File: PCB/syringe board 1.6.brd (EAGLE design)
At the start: 68.6 x 30.5 mm, 40 parts, among them IC1 A3967SLB, Q1 RESONATOR_CSTCE_V, U1 ATMEGA328P_TQFP, U2 PCA9306

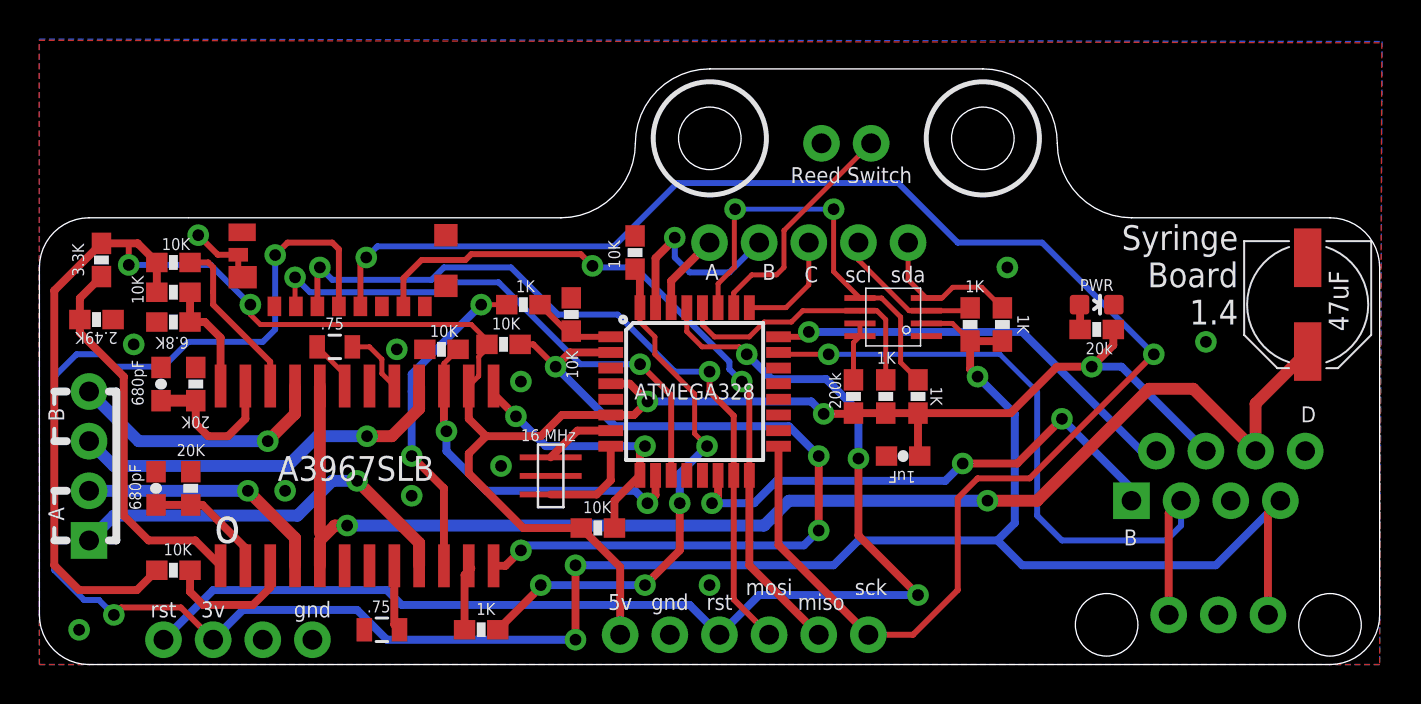
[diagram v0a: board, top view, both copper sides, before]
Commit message: PCB update to 1.6
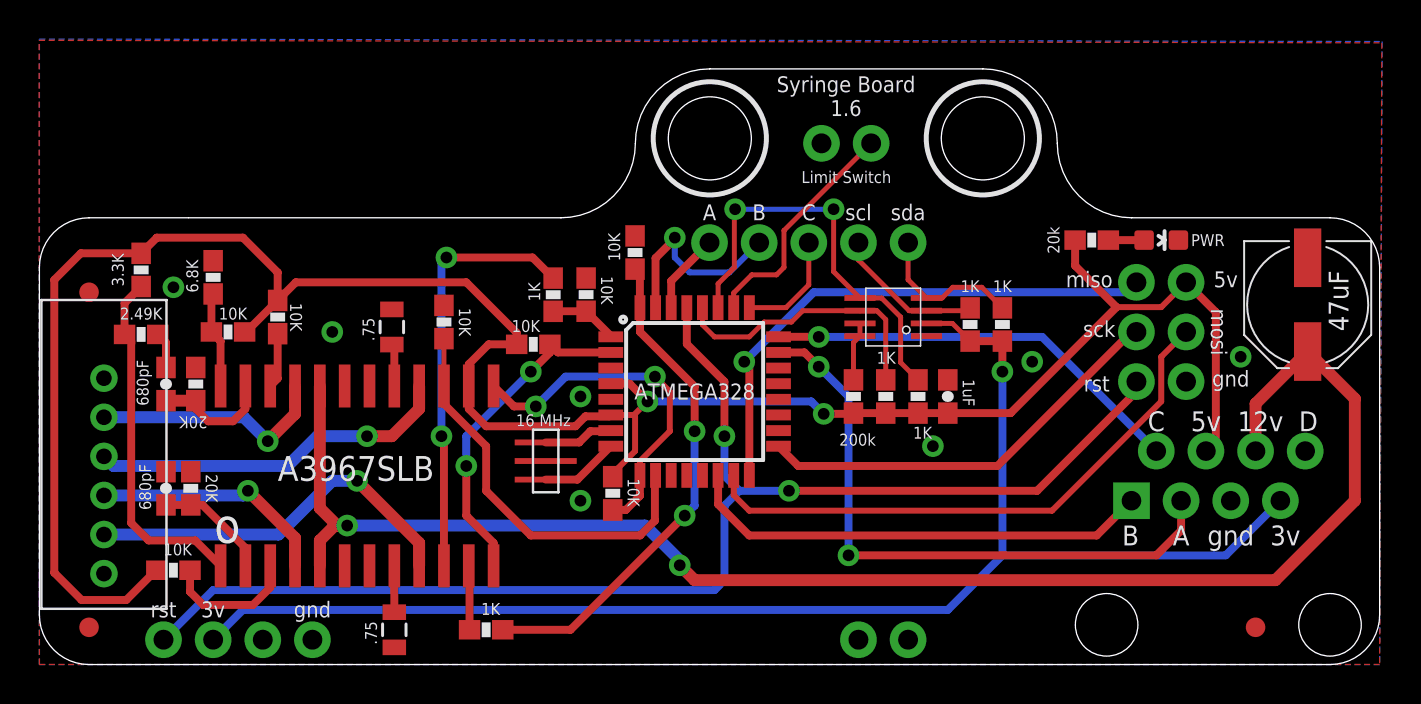
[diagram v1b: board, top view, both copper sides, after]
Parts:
- removed C5: 680pF, SparkFun-Capacitors:0603-CAP
- removed JP1: (no value), SparkFun-Connectors:1X06_NO_SILK
- removed JP3: (no value), SparkFun:1X04_NO_SILK
- removed JP6: (no value), SparkFun-Connectors:1X03_NO_SILK
- removed PWR: (no value), Andy-library:LED-0603
- added C1: 680pF, SparkFun-Capacitors:0603-CAP
- added J1: RJ45, Andy-library:RJ45-8
- added J2: AVR_SPI_PROG_3X2NS, SparkFun-Connectors:2X3-NS
- added J5: (no value), SparkFun-Connectors:1X02_NO_SILK
- added LED1: PWR, Andy-library:LED-0603
- added U$3: FIDUCIAL, adafruit:FIDUCIAL_1MM
- added U$5: OMRON_4PIN, Andy-library:OMRON_4PIN
- JP2: device SparkFun-Connectors:1X05_NO_SILK -> SparkFun-Connectors:1X04_NO_SILK_ALL_ROUND
- JP4: device SparkFun-Connectors:1X04_NO_SILK_ALL_ROUND -> SparkFun-Connectors:1X05_NO_SILK
- JP5: device SparkFun-Connectors:1X02_NO_SILK -> SparkFun-Connectors:1X02_NO_SILK@1
- R1: value .75 -> 3.3K; device SparkFun-Resistors:0805 -> SparkFun-Resistors:0603-RES
- R16: value 3.3K -> 10K
- R17: value 6.8K -> 1K
- R2: value .75 -> 2.49K; device SparkFun-Resistors:0805 -> SparkFun-Resistors:0603-RES
- R20: value 10K -> 1K
- R21: value 10K -> 200k
- R23: value 20k -> 1K
- R4: value 20K -> 20k
- R5: value 2.49K -> .75; device SparkFun-Resistors:0603-RES -> SparkFun-Resistors:0805
- R6: value 200k -> .75; device SparkFun-Resistors:0603-RES -> SparkFun-Resistors:0805
- R7: value 1K -> 10K
- R8: value 1K -> 20K
- R9: value 1K -> 6.8K
- U$1: value MICROSD_SOCKET -> FIDUCIAL; device Andy-library:MICROSD -> adafruit:FIDUCIAL_1MM
- U$2: value RJ45 -> FIDUCIAL; device Andy-library:RJ45-8 -> adafruit:FIDUCIAL_1MM
- moved U$2 57.8 mm to (2.54, 1.91)
- moved R4 46.4 mm to (53.8, 21.7), turned to 0 degrees
- moved R17 42.4 mm to (49.3, 17.4), turned to 90 degrees
- moved R9 40.5 mm to (8.89, 19.8), turned to 270 degrees
- moved R8 37.0 mm to (8.00, 14.4), turned to 270 degrees
- moved JP2 34.5 mm to (6.35, 1.27)
- moved JP4 34.5 mm to (34.3, 21.6)
- moved R7 33.8 mm to (9.65, 17.0), turned to 0 degrees
- moved R16 24.9 mm to (28.0, 18.9), turned to 270 degrees
- moved R6 23.9 mm to (18.0, 17.3), turned to 270 degrees
- moved R1 22.2 mm to (5.21, 20.2), turned to 90 degrees
- moved R5 22.0 mm to (18.2, 1.78), turned to 90 degrees
- moved R12 18.6 mm to (25.3, 16.4)
- moved R20 17.5 mm to (47.6, 17.4), turned to 90 degrees
- moved R21 15.0 mm to (41.7, 13.7), turned to 90 degrees
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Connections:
- removed net MISO: JP1.5, U$1.P7, U1.16
- removed net MOSI: JP1.4, U$1.P3, U1.15
- removed net N$13: U1.12
- removed net SCK: JP1.6, U$1.P5, U1.17
- new net N$10: J2.3, U1.17
- net 12VDC: now also J1.6; no longer U$2.6
- net 3VDC: now also J1.7, JP2.2, R17.1, R20.1; no longer JP4.2, JP6.1, R22.1, R9.1, U$1.P4, U$2.7
- net 5VDC: now also J1.4, J2.2, R1.2, R13.2, R21.1, R22.1, R4.1, R7.2; no longer JP1.1, R10.2, R15.2, R16.2, R6.1, R7.1, R8.1, U$2.4
- net DIR_IN: now also R10.2; no longer R20.2
- net DISP_SCL: now also JP4.4, R20.2; no longer JP2.4, R22.2
- net DISP_SDA: now also JP4.5, R17.2; no longer JP2.5, R9.2
- net ENABLE: now also R15.2; no longer R13.2
- net GND: now also C1.2, J1.5, J2.6, JP2.4, LED1.C, R10.1, R15.1, R16.1, R6.1, R8.1, R9.1, U$5.G1, U$5.G2; no longer C5.2, JP1.2, JP4.4, JP6.2, PWR.C, R1.1, R13.1, R17.1, R20.1, R21.1, R4.1, U$1.G1, U$1.G2, U$1.G3, U$1.G4, U$1.P6, U$2.5
- net MCU_SCL: now also R22.2; no longer R7.2
- net MCU_SDA: now also R23.2; no longer R8.2
- net MS1: now also R12.1; no longer R14.1
- net MS2: now also R13.1; no longer R10.1
- net N$1: now also R5.2; no longer R1.2
- net N$11: now also J2.4, U1.15; no longer U1.13
- net N$12: now also J1.3; no longer JP6.3, U$2.3
- net N$15: now also JP4.1; no longer JP2.1
- net N$16: now also JP4.2; no longer JP2.2
- net N$17: now also JP4.3; no longer JP2.3
- net N$20: now also J1.2; no longer U$2.2
- net N$21: now also J1.1; no longer U$2.1
- net N$3: now also R6.2; no longer R2.2
- net N$5: now also C1.1; no longer C4.1
- net N$6: now also R21.2; no longer R6.2
- net N$7: now also C4.1, R8.2; no longer C5.1, R4.2
- net N$8: now also LED1.A, R4.2; no longer PWR.A, R23.2
- net N$9: now also J2.1, U1.16; no longer U$1.P2, U1.11
- net OUT1A: now also U$5.2; no longer JP3.3
- net OUT1B: now also U$5.1; no longer JP3.4
- net OUT2A: now also U$5.4; no longer JP3.1
- net OUT2B: now also U$5.3; no longer JP3.2
- net PFD: now also R7.1, R9.2; no longer R12.1, R17.2
- net RESET: now also R14.1; no longer R15.1
- net RST: now also J2.5, JP2.1; no longer JP1.3, JP4.1
- net STEP_IN: now also R16.2; no longer R21.2
- net VREF: now also R1.1, R2.2; no longer R16.1, R5.2
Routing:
- net SCK: track 83.0 -> 0.00 mm, vias 2 -> 0
- net 3VDC: track 127.0 -> 72.8 mm, vias 5 -> 1
- net MOSI: track 39.4 -> 0.00 mm, vias 2 -> 0
- net MISO: track 36.8 -> 0.00 mm, vias 2 -> 0
- net N$11: track 0.00 -> 29.6 mm
- net MS1: track 42.0 -> 17.0 mm, vias 4 -> 2
- net N$10: track 0.00 -> 21.6 mm
- net 12VDC: track 67.8 -> 79.9 mm
- net RESET: track 8.57 -> 2.84 mm
- net STEP: track 16.8 -> 21.8 mm
- net RST: track 63.8 -> 68.3 mm, vias 3 -> 2
- net N$12: track 36.0 -> 31.7 mm, vias 1 -> 2
- net MS2: track 14.1 -> 18.1 mm
- net GND: track 6.29 -> 2.46 mm, vias 11 -> 7
- net N$21: track 26.9 -> 24.0 mm, vias 3 -> 0
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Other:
- board text added: "Limit Switch"
- board text added: "Syringe Board 1.6"
- board text removed: "Reed Switch"
- board text removed: "Syringe Board 1.4"
